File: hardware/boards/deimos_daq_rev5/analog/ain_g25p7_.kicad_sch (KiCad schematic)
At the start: 6 parts, among them IC38001 INA826AIDR

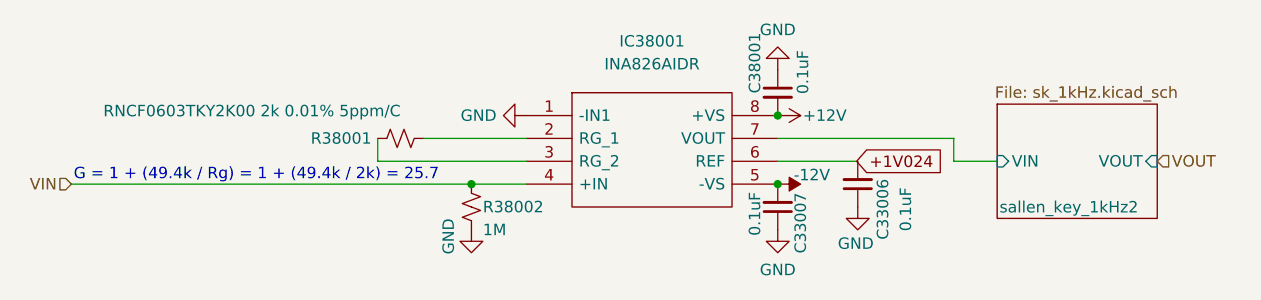
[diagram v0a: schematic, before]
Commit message: restore rev5 and make this rev rev6
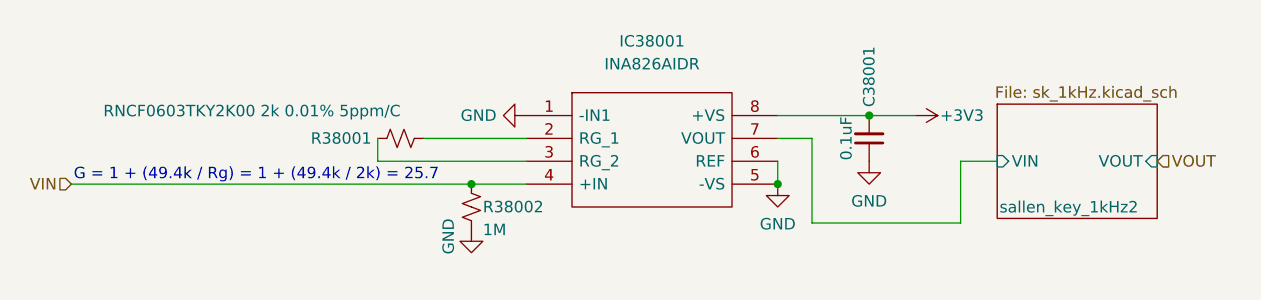
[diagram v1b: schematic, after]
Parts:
- removed C33006, C33007: 0.1uF, Capacitor_SMD:C_0402_1005Metric, symbol Device:C_Small
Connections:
- net +1V024 is gone; now on net GND: IC38001.6 (REF)
- net -12V is gone; now on net GND: IC38001.5 (-VS)
- net +12V renamed +3V3
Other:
- moved on the sheet: C38001
